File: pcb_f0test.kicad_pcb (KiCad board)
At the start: 2 copper layers, 50 x 6 mm, 36 parts, among them P1 CONN_02X04, P2 CONN_01X02, U1 STM32F042GxU, U2 LP2985LV

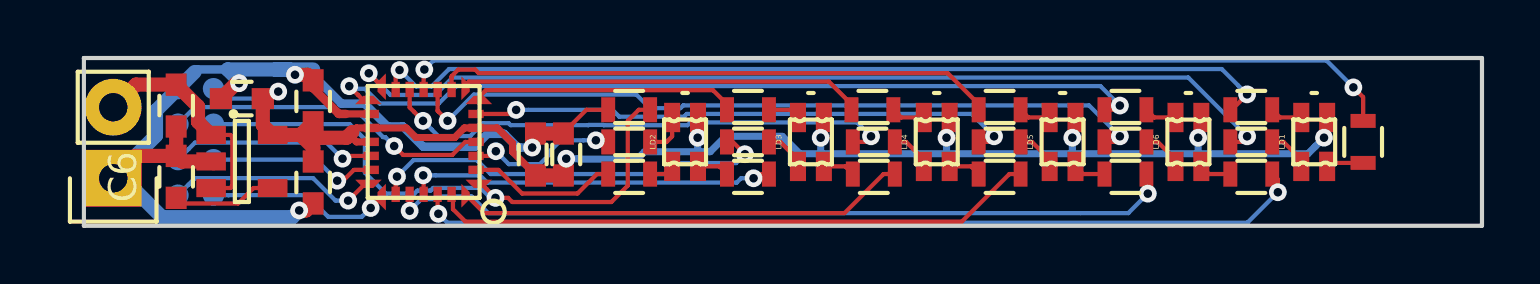
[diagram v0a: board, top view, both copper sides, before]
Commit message: Fairly good routing now.
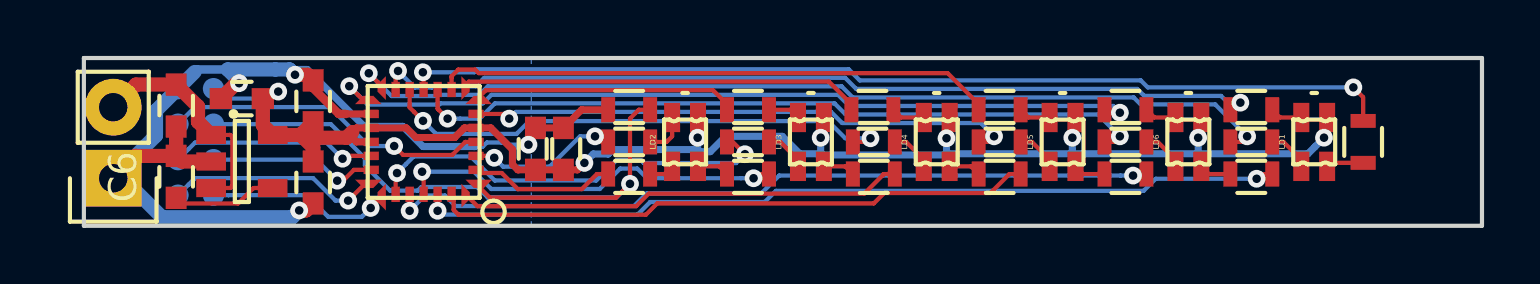
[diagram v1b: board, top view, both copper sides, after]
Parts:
- moved C2 0.20 mm to (43.1, 63.2)
- moved C4 0.20 mm to (44.1, 63.2)
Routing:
- net /boot0: track 21.3 -> 25.5 mm
- net /ldr6: track 32.0 -> 31.1 mm
- net /ldb1: track 32.8 -> 32.0 mm
- net /ldr2: track 13.3 -> 14.0 mm
- net /ldr5: track 28.5 -> 27.8 mm
- net +3V3: track 56.4 -> 55.8 mm
- added copper zone on B.Cu, net +3V3

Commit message: Some misc. changes.
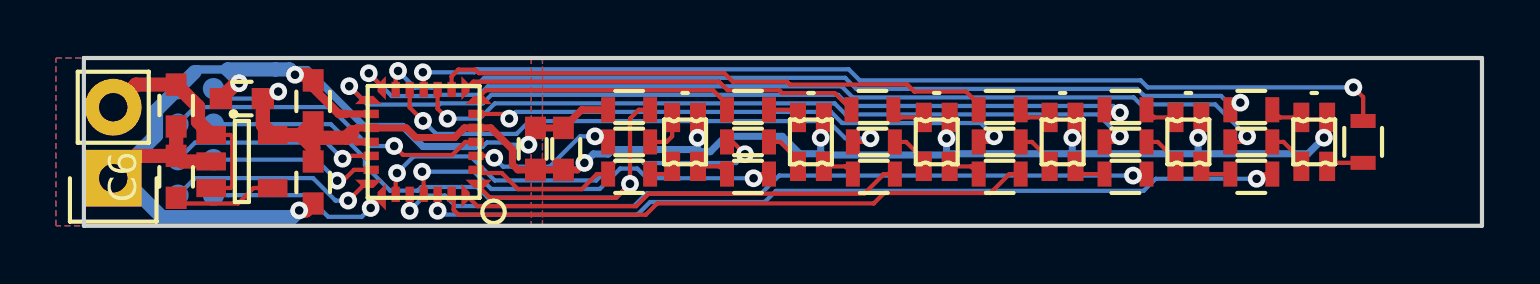
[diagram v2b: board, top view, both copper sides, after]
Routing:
- added copper zone on F.Cu, net +3V3
- added copper zone on B.Cu, net GND
- added copper zone on F.Cu, net GND
